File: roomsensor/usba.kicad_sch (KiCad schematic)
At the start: 4 parts, among them U801 USBLC6-2SC6

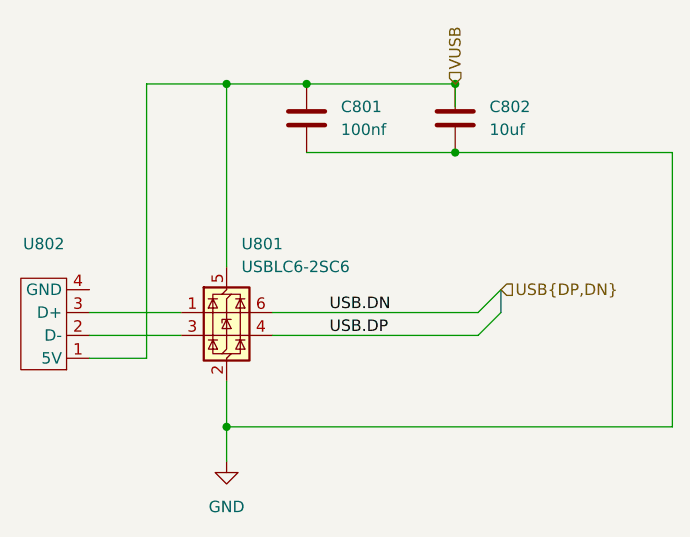
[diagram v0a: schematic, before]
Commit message: more work on roomsensor
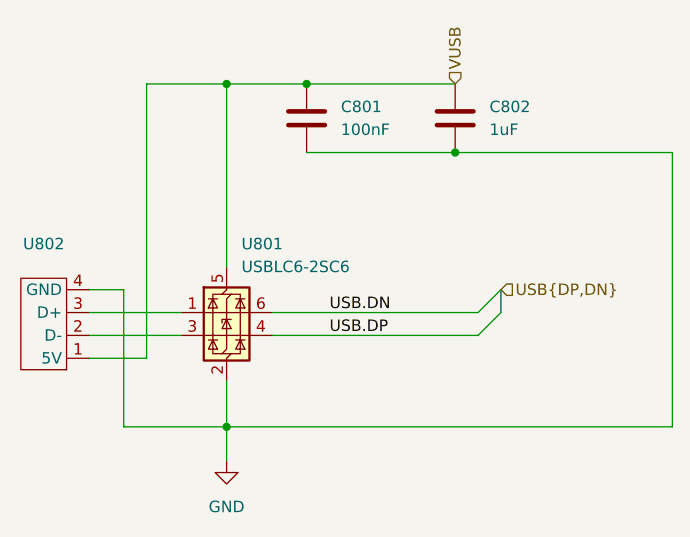
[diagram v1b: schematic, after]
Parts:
- C801: value 100nf -> 100nF
- C802: value 10uf -> 1uF
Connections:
- net GND: now also U802.4 (GND)
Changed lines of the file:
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@@
+	)
+	(junction
+		(at 133.35 83.82)
+		(diameter 0)
+		(color 0 0 0 0)
 	)
 	(junction
@@
 	)
 	(junction
-		(at 133.35 83.82)
-		(diameter 0)
-		(color 0 0 0 0)
-	)
-	(junction
 		(at 142.24 83.82)
 		(diameter 0)
 		(color 0 0 0 0)
 	)
-	(junction
-		(at 158.75 83.82)
-		(diameter 0)
-		(color 0 0 0 0)
-	)
 	(bus_entry
 		(at 163.83 106.68)
@@
 	(wire
 		(pts
+			(xy 118.11 106.68) (xy 121.92 106.68)
+		)
+		(stroke
+			(width 0)
+			(type default)
+		)
+	)
+	(wire
+		(pts
+			(xy 121.92 106.68) (xy 121.92 121.92)
+		)
+		(stroke
+			(width 0)
+			(type default)
+		)
+	)
+	(wire
+		(pts
 			(xy 124.46 83.82) (xy 133.35 83.82)
 		)
@@
 	(wire
 		(pts
-			(xy 158.75 83.82) (xy 158.75 86.36)
+			(xy 121.92 121.92) (xy 133.35 121.92)
 		)
 		(stroke
@@
 	(wire
 		(pts
-			(xy 182.88 91.44) (xy 158.75 91.44)
-		)
-		(stroke
-			(width 0)
-			(type default)
-		)
-	)
-	(wire
-		(pts
 			(xy 182.88 121.92) (xy 182.88 91.44)
 		)
@@
 		(pts
 			(xy 133.35 121.92) (xy 182.88 121.92)
+		)
+		(stroke
+			(width 0)
+			(type default)
+		)
+	)
+	(wire
+		(pts
+			(xy 158.75 91.44) (xy 182.88 91.44)
 		)
 		(stroke
@@
 	)
 	(symbol
+		(lib_id "Device:C")
+		(at 158.75 87.63 0)
+		(unit 1)
+		(exclude_from_sim no)
+		(in_bom yes)
+		(on_board yes)
+		(dnp no)
+		(fields_autoplaced yes)
+		(property "Reference" "C802"
+			(at 162.56 86.3599 0)
+			(effects
+				(font
+					(size 1.27 1.27)
+				)
+				(justify left)
+			)
+		)
+		(property "Value" "1uF"
+			(at 162.56 88.8999 0)
+			(effects
+				(font
+					(size 1.27 1.27)
+				)
+				(justify left)
+			)
+		)
+		(property "Footprint" "Capacitor_SMD:C_0603_1608Metric"
+			(at 159.7152 91.44 0)
+			(effects
+				(font
+					(size 1.27 1.27)
+				)
+				(hide yes)
+			)
+		)
+		(property "Datasheet" "~"
+			(at 158.75 87.63 0)
+			(effects
+				(font
+					(size 1.27 1.27)
+				)
+				(hide yes)
+			)
+		)
+		(property "Description" "Unpolarized capacitor"
+			(at 158.75 87.63 0)
+			(effects
+				(font
+					(size 1.27 1.27)
+				)
+				(hide yes)
+			)
+		)
+		(pin "1"
+		)
+		(pin "2"
+		)
+		(instances
+			(project "roomsensor"
+				(path "/48ddfdd8-68fa-4e63-aa18-bc113cdf8cfa/acb10ddb-98c9-439e-a93d-9b153e35464d"
+					(reference "C802")
+					(unit 1)
+				)
+			)
+		)
+	)
+	(symbol
 		(lib_id "power:GND")
 		(at 133.35 125.73 0)
@@
 				(path "/48ddfdd8-68fa-4e63-aa18-bc113cdf8cfa/acb10ddb-98c9-439e-a93d-9b153e35464d"
 					(reference "#PWR0802")
-					(unit 1)
-				)
-			)
-		)
-	)
-	(symbol
-		(lib_id "Device:C")
-		(at 158.75 87.63 0)
-		(unit 1)
-		(exclude_from_sim no)
-		(in_bom yes)
-		(on_board yes)
-		(dnp no)
-		(fields_autoplaced yes)
-		(property "Reference" "C802"
-			(at 162.56 86.3599 0)
-			(effects
-				(font
-					(size 1.27 1.27)
-				)
-				(justify left)
-			)
-		)
-		(property "Value" "10uf"
-			(at 162.56 88.8999 0)
-			(effects
-				(font
-					(size 1.27 1.27)
-				)
-				(justify left)
-			)
-		)
-		(property "Footprint" "Capacitor_SMD:C_0603_1608Metric"
-			(at 159.7152 91.44 0)
-			(effects
-				(font
-					(size 1.27 1.27)
-				)
-				(hide yes)
-			)
-		)
-		(property "Datasheet" "~"
-			(at 158.75 87.63 0)
-			(effects
-				(font
-					(size 1.27 1.27)
-				)
-				(hide yes)
-			)
-		)
-		(property "Description" "Unpolarized capacitor"
-			(at 158.75 87.63 0)
-			(effects
-				(font
-					(size 1.27 1.27)
-				)
-				(hide yes)
-			)
-		)
-		(pin "1"
-		)
-		(pin "2"
-		)
-		(instances
-			(project "roomsensor"
-				(path "/48ddfdd8-68fa-4e63-aa18-bc113cdf8cfa/acb10ddb-98c9-439e-a93d-9b153e35464d"
-					(reference "C802")
 					(unit 1)
 				)
@@
 			)
 		)
-		(property "Value" "100nf"
+		(property "Value" "100nF"
 			(at 146.05 88.8999 0)
 			(effects
